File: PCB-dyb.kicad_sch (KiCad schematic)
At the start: 5 parts, among them U1 74AUC2G08, U2 74AUC2G08, U3 74AUC2G04, U4 74AUC2G04, U5 74AUC2G04

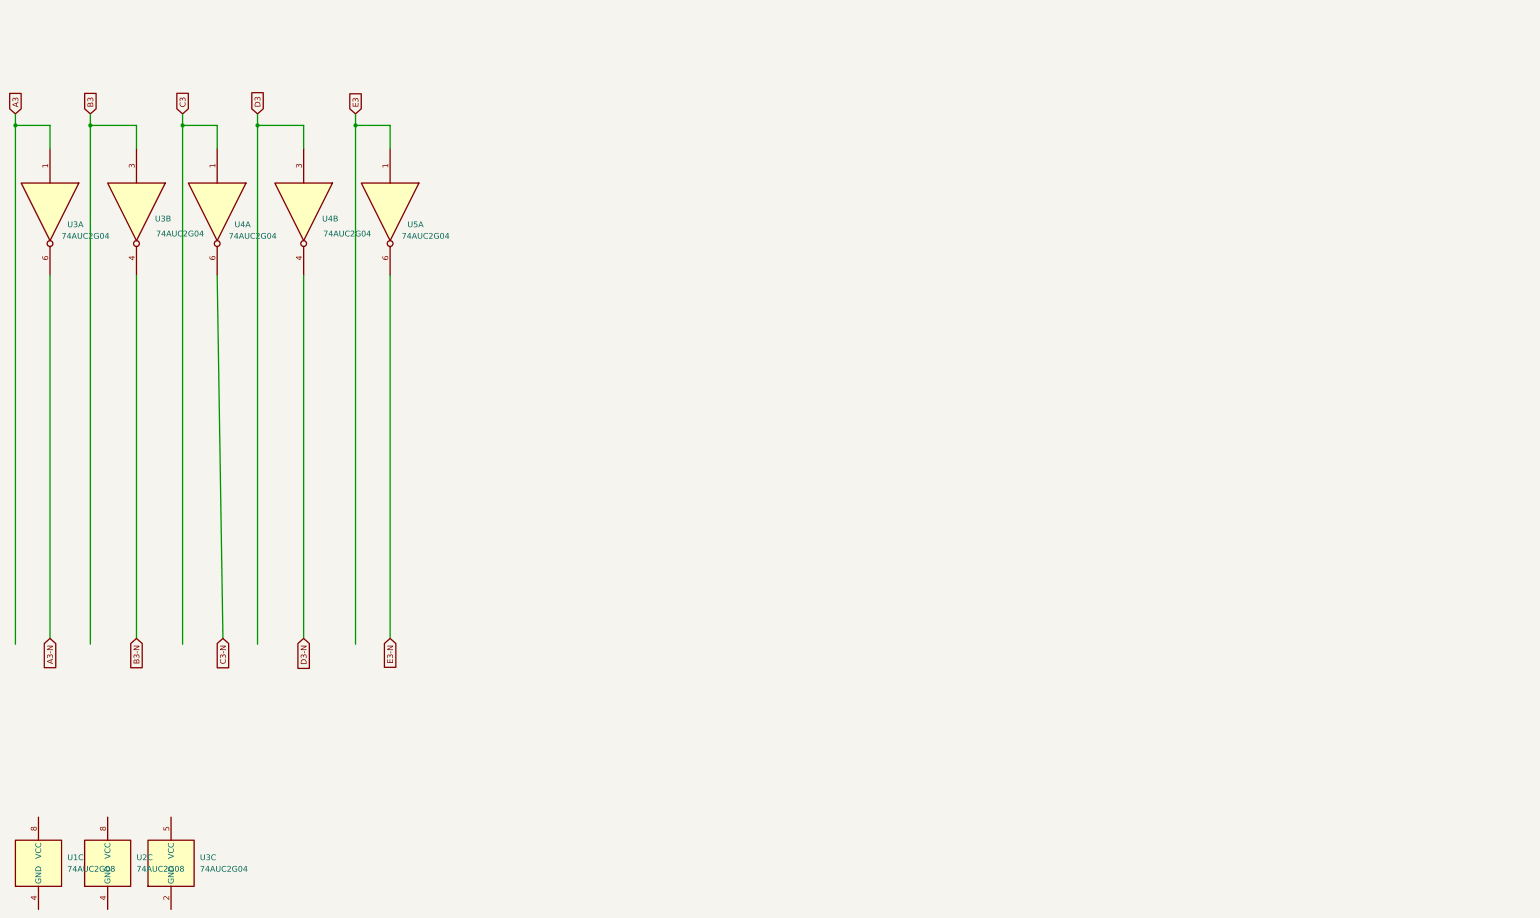
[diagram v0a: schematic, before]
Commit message: Somme 2*4bits
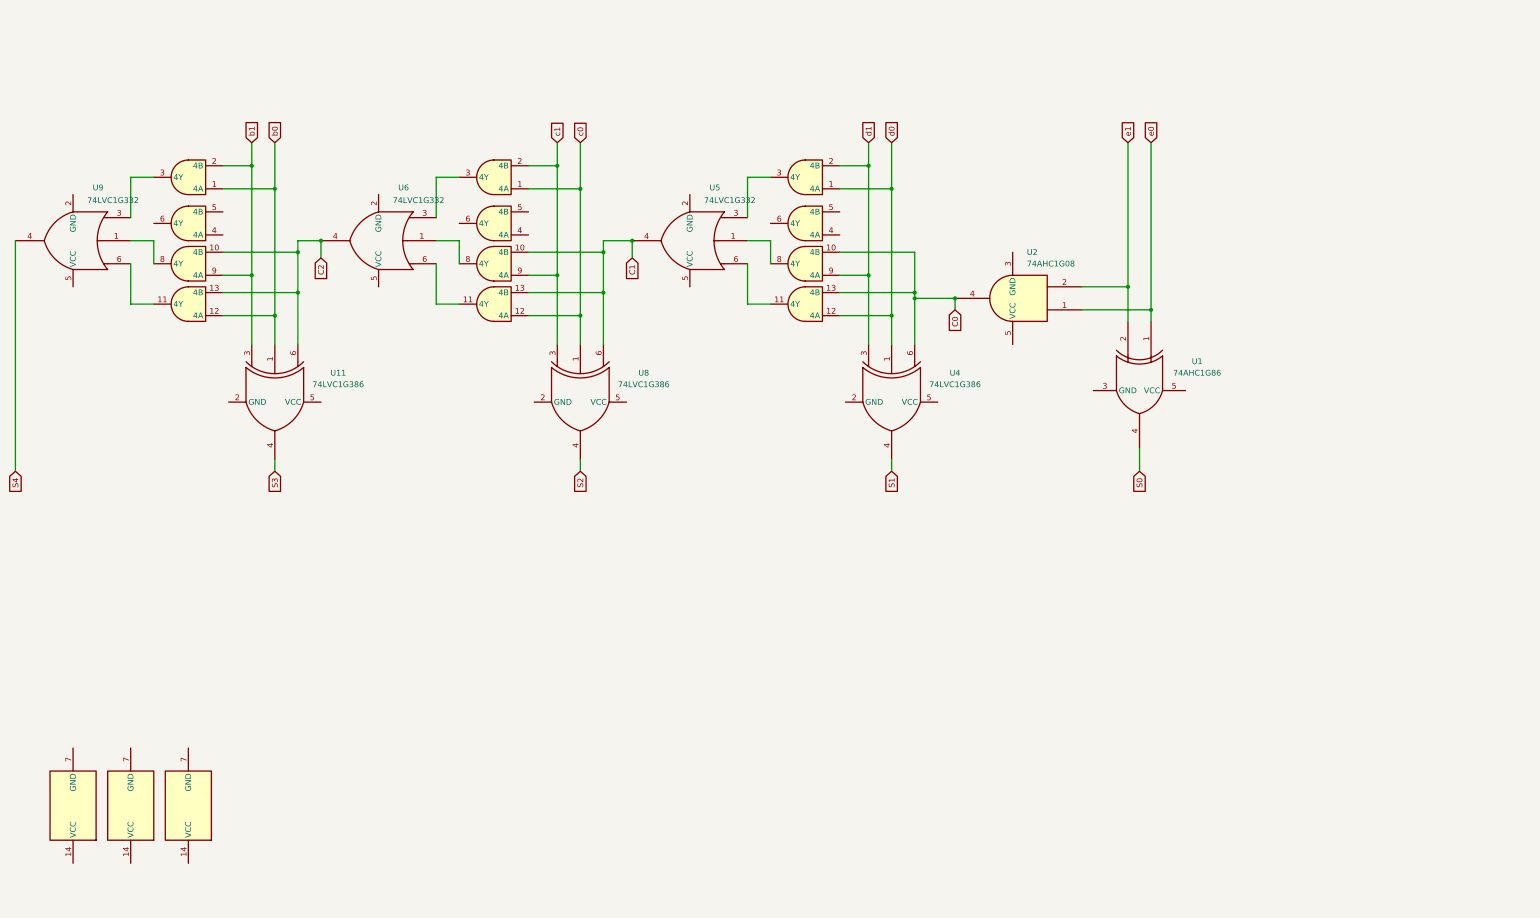
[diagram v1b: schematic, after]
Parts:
- removed U1, U2: 74AUC2G08, symbol 74xGxx:74AUC2G08
- removed U3, U4, U5: 74AUC2G04, symbol 74xGxx:74AUC2G04
- added U1: 74AHC1G86, symbol 74xGxx:74AHC1G86
- added U10, U3, U7: (no value), Package_Sorën:SOIC-14_3.9x8.7mm_P1.27mm, symbol CornetPrisme_Library:SN74ALVC08DR
- added U11, U4, U8: 74LVC1G386, symbol 74xGxx:74LVC1G386
- added U2: 74AHC1G08, symbol 74xGxx:74AHC1G08
- added U5, U6, U9: 74LVC1G332, symbol 74xGxx:74LVC1G332
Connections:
- new net: U6.3, U7.3 (4Y)
- new net: U6.6, U7.11 (4Y)
- new net: U10.8 (4Y), U9.1
- new net: U10.3 (4Y), U9.3
- new net: U10.11 (4Y), U9.6
- new net: U6.1, U7.8 (4Y)
- new net: U3.8 (4Y), U5.1
- new net: U3.3 (4Y), U5.3
- new net: U3.11 (4Y), U5.6
- new net C0: U2.4, U3.10 (4B), U3.13 (4B), U4.6
- new net C1: U5.4, U7.10 (4B), U7.13 (4B), U8.6
- new net C2: U10.10 (4B), U10.13 (4B), U11.6, U6.4
- new net S0: U1.4
- new net S1: U4.4
- new net S2: U8.4
- new net S3: U11.4
- new net S4: U9.4
- new net b0: U10.1 (4A), U10.12 (4A), U11.1
- new net b1: U10.2 (4B), U10.9 (4A), U11.3
- new net c0: U7.1 (4A), U7.12 (4A), U8.1
- new net c1: U7.2 (4B), U7.9 (4A), U8.3
- new net d0: U3.1 (4A), U3.12 (4A), U4.1
- new net d1: U3.2 (4B), U3.9 (4A), U4.3
- new net e0: U1.1, U2.1
- new net e1: U1.2, U2.2

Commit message: Add : adder logic
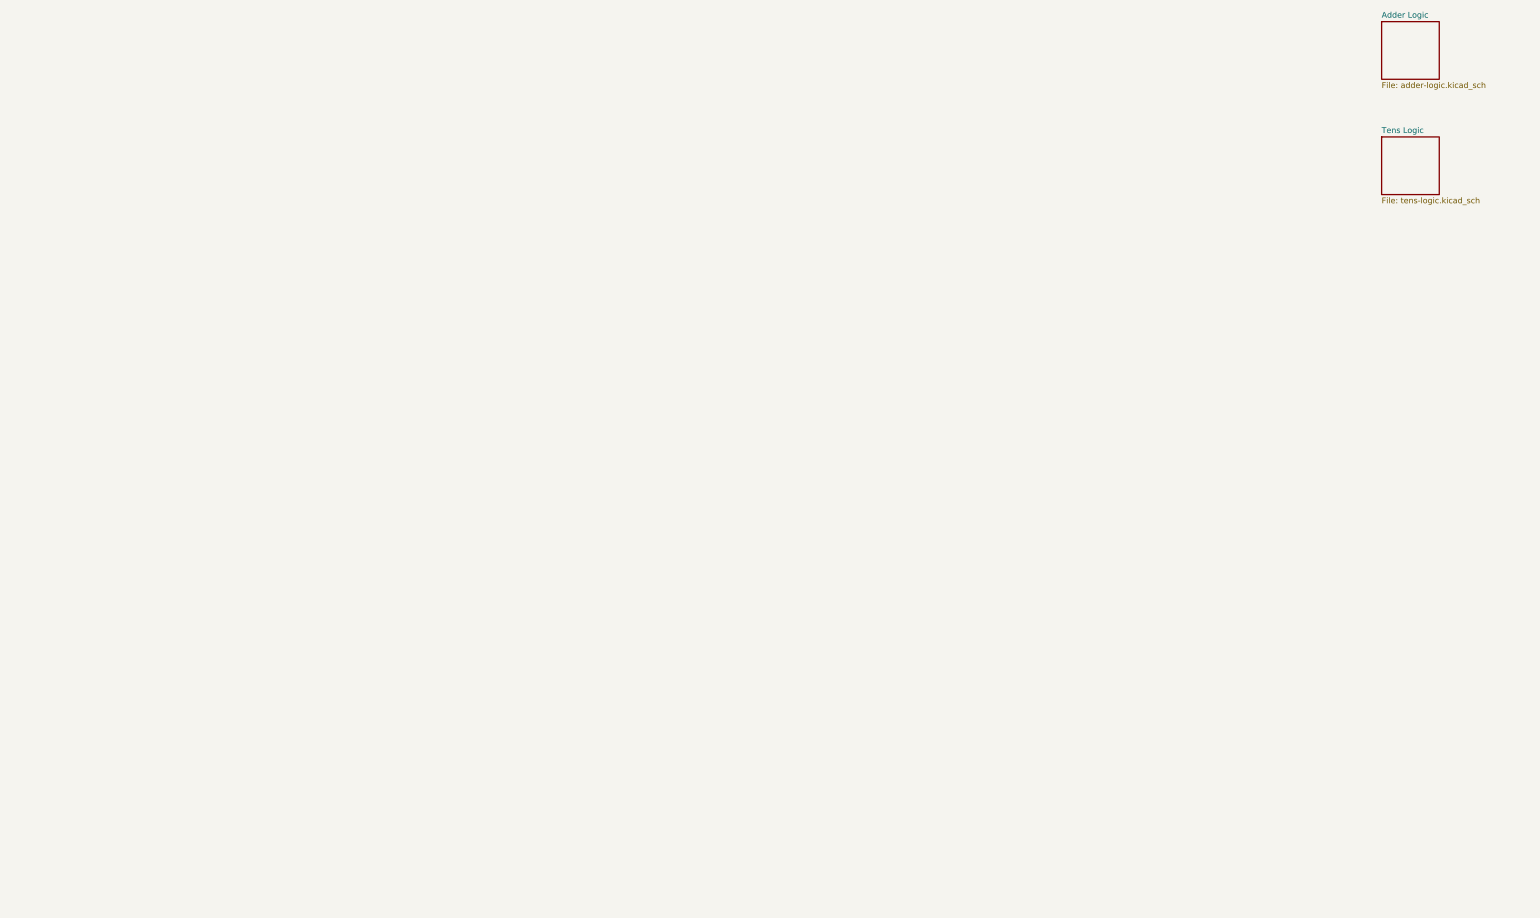
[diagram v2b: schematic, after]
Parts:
- removed U1: 74AHC1G86, symbol 74xGxx:74AHC1G86
- removed U10, U3, U7: (no value), Package_Sorën:SOIC-14_3.9x8.7mm_P1.27mm, symbol CornetPrisme_Library:SN74ALVC08DR
- removed U11, U4, U8: 74LVC1G386, symbol 74xGxx:74LVC1G386
- removed U2: 74AHC1G08, symbol 74xGxx:74AHC1G08
- removed U5, U6, U9: 74LVC1G332, symbol 74xGxx:74LVC1G332
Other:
- added sheet Adder Logic (adder-logic.kicad_sch)
- added sheet Tens Logic (tens-logic.kicad_sch)
